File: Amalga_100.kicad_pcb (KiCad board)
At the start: 6 copper layers, 268 x 155 mm, 223 parts, among them IC1 ADM3052, IC3 INA240A1, IC4 INA240A1, IC5 INA240A1, P1 USB_B, P10 IN-, P2 Interface, P3 IN+, P4 IN-, P5 MOTOR3, P6 MOTOR2, P7 MOTOR1, P8 SWD, P9 CONN_6-HSWR-V2-rescue, Q1 IRFP4668PBF, Q10 IRFP4668PBF, Q11 IRFP4668PBF, Q12 IRFP4668PBF, Q2 IRFP4668PBF, Q3 IRFP4668PBF, Q4 IRFP4668PBF, Q5 IRFP4668PBF, Q6 IRFP4668PBF, Q7 IRFP4668PBF, Q8 IRFP4668PBF, Q9 IRFP4668PBF, SW1 SW_DIP_x02, U1 STM32F40X_LQFP64, U10 AD8397, U11 ADM811, U2 B1215S-2W, U3 JW5052C, U4 JW5052C, U5 ADUM3160, U6 AD2S1205, U7 IRS2186, U8 IRS2186, U9 IRS2186, Y1 8MHz, Y2 8.912 MHZ

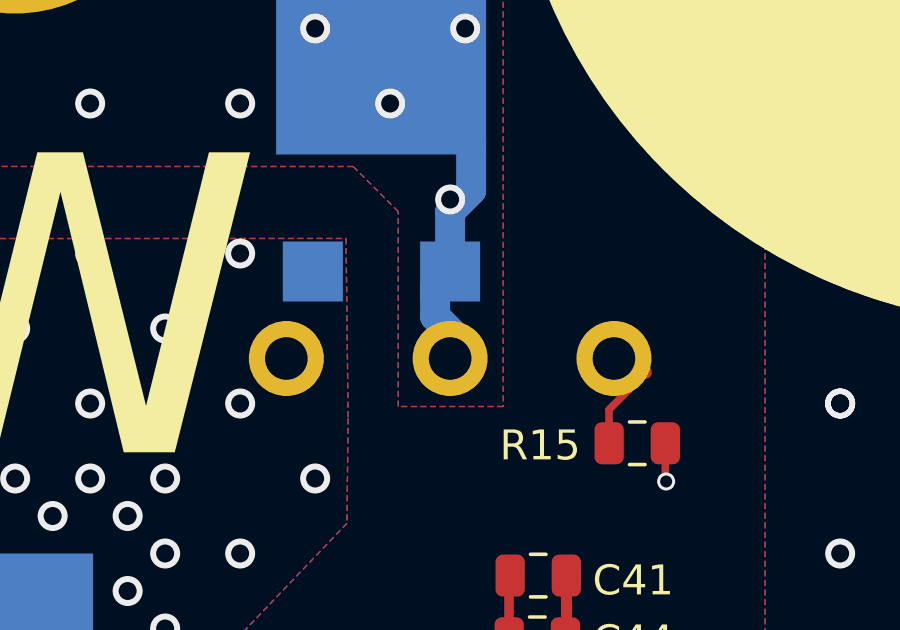
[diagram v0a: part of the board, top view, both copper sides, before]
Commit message: BU
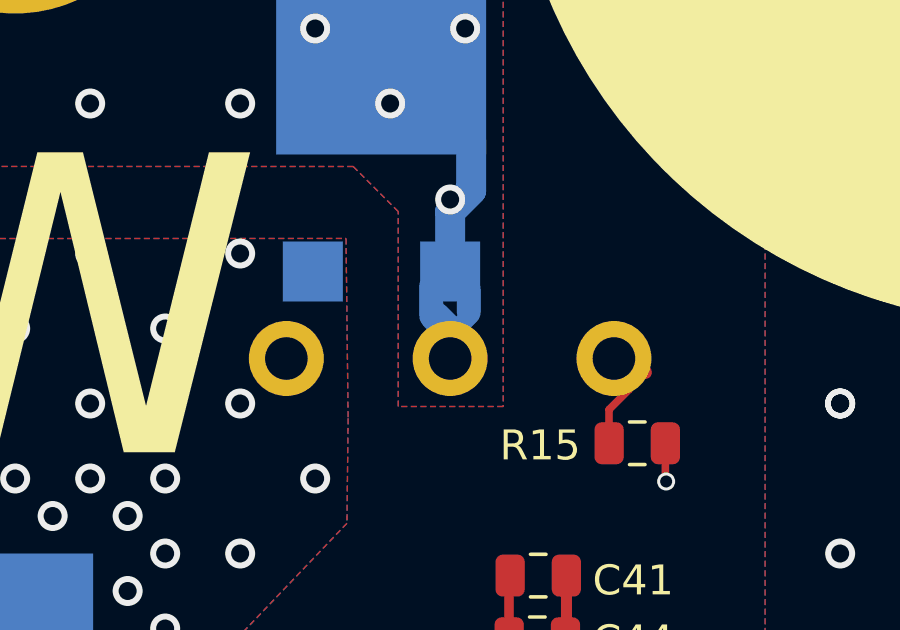
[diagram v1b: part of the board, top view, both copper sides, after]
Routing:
- net H1_VS: track 166.4 -> 169.8 mm
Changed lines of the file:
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@@
     (thickness 1.6)
     (drawings 85)
-    (tracks 4039)
+    (tracks 4043)
     (zones 0)
     (modules 223)
@@
   (page A4)
   (layers
-    (0 "F.Cu_(top)" signal hide)
+    (0 "F.Cu_(top)" signal)
     (1 inner_layer1 power hide)
     (2 inner_layer2 power hide)
@@
   )
   (setup
-    (last_trace_width 0.3)
+    (last_trace_width 0.6)
     (user_trace_width 0.2)
     (user_trace_width 0.25)
@@
   (segment (start 245.71 73.41) (end 244.9 72.6) (width 1) (layer "B.Cu_(GND_bottom)") (net 98))
   (segment (start 244.9 71.6) (end 245.4 71.1) (width 1) (layer "B.Cu_(GND_bottom)") (net 98))
-  (segment (start 244.9 72.6) (end 244.9 71.6) (width 1) (layer "B.Cu_(GND_bottom)") (net 98))
+  (segment (start 244.77 72.58) (end 244.77 71.58) (width 0.8) (layer "B.Cu_(GND_bottom)") (net 98))
   (segment (start 246.1 68.4) (end 246.1 66.7) (width 1) (layer "B.Cu_(GND_bottom)") (net 98))
   (segment (start 245.4 71.1) (end 245.4 69.1) (width 1) (layer "B.Cu_(GND_bottom)") (net 98))
@@
   (segment (start 240.9 42.3) (end 240.8 42.2) (width 0.6) (layer "F.Cu_(top)") (net 98))
   (segment (start 240.8 42.2) (end 240.8 41.3) (width 0.6) (layer "F.Cu_(top)") (net 98))
+  (segment (start 245.4 74) (end 245.4 73.23) (width 0.6) (layer "B.Cu_(GND_bottom)") (net 98))
+  (segment (start 245.4 73.23) (end 246.09 72.54) (width 0.6) (layer "B.Cu_(GND_bottom)") (net 98))
+  (segment (start 246.09 71.79) (end 245.4 71.1) (width 0.6) (layer "B.Cu_(GND_bottom)") (net 98))
+  (segment (start 246.02 72.45) (end 246.02 71.7) (width 0.8) (layer "B.Cu_(GND_bottom)") (net 98))
   (via (at 49.9 75) (size 0.6) (drill 0.4) (layers "F.Cu_(top)" "B.Cu_(GND_bottom)") (net 99))
   (segment (start 44.187351 76.312649) (end 44.574999 75.925001) (width 0.45) (layer "B.Cu_(GND_bottom)") (net 99))
